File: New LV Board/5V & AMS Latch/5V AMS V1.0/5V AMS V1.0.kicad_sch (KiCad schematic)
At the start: 16 parts, among them J2 B12B-PH-K-S, J4 691137710002, K2 A161CS12VDC.64, K3 A161CS12VDC.64, K4 A161CS12VDC.64, SW1 Test Reset AMS, U1 LT1117-5.0

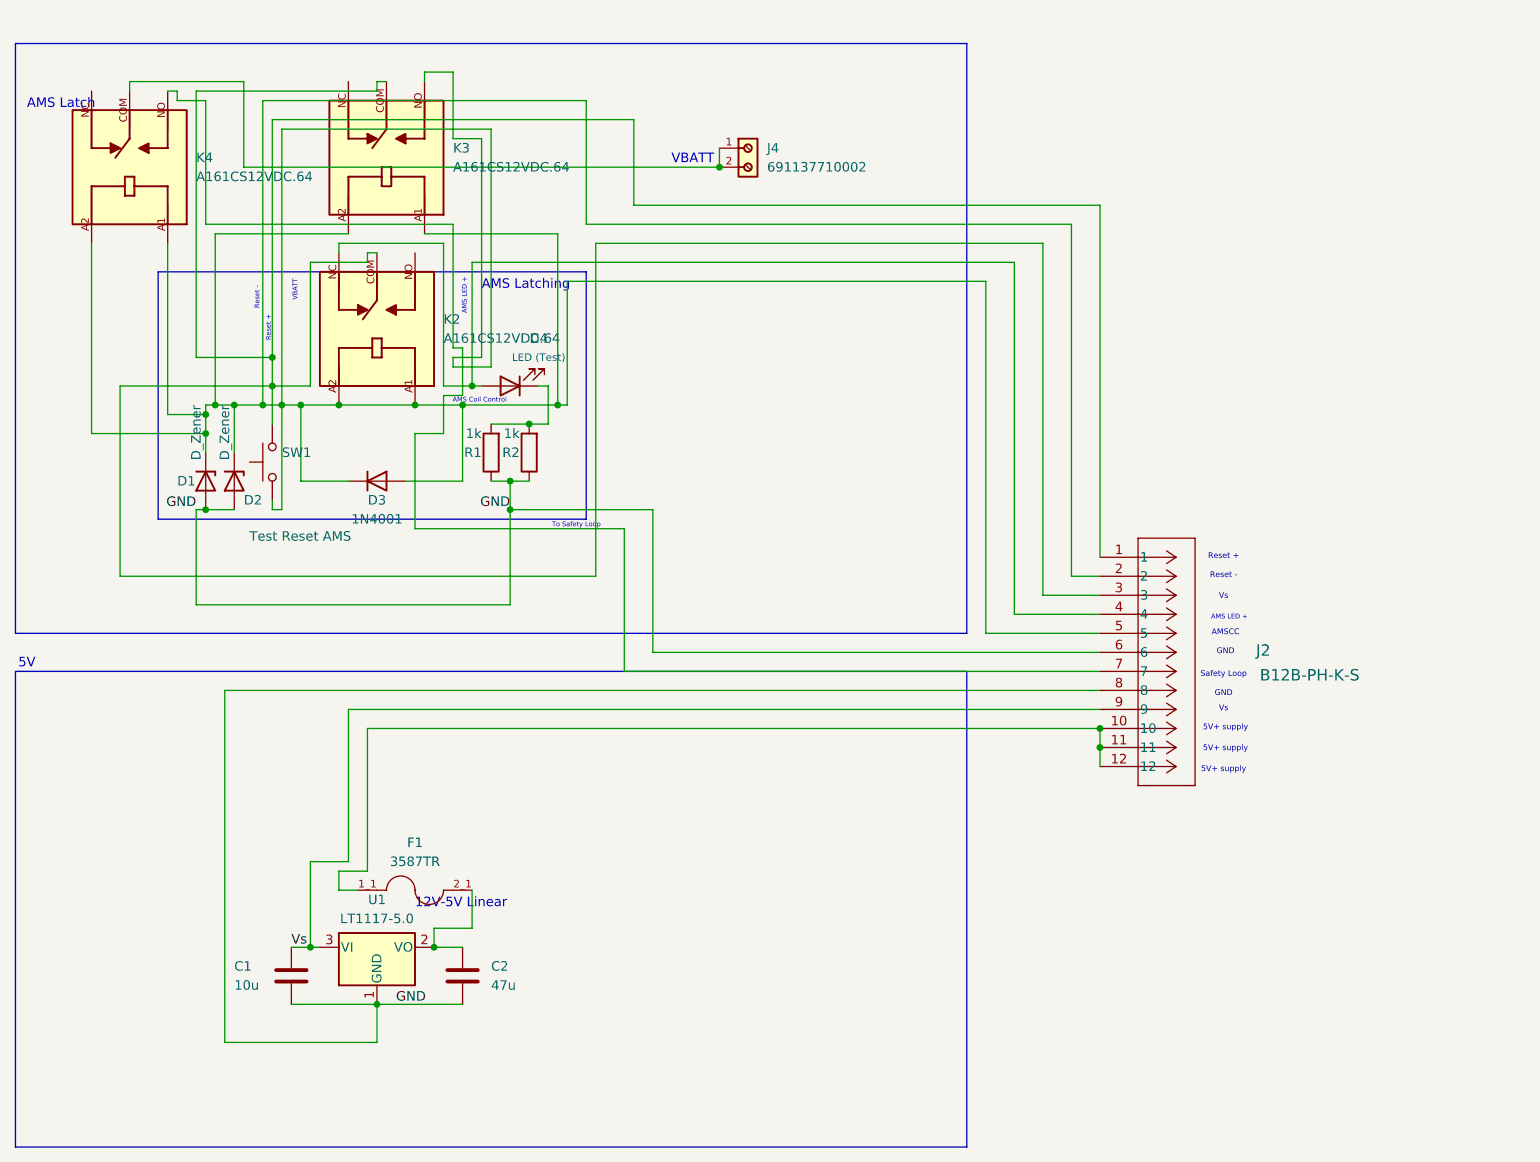
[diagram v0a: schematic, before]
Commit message: cleaned up schematics
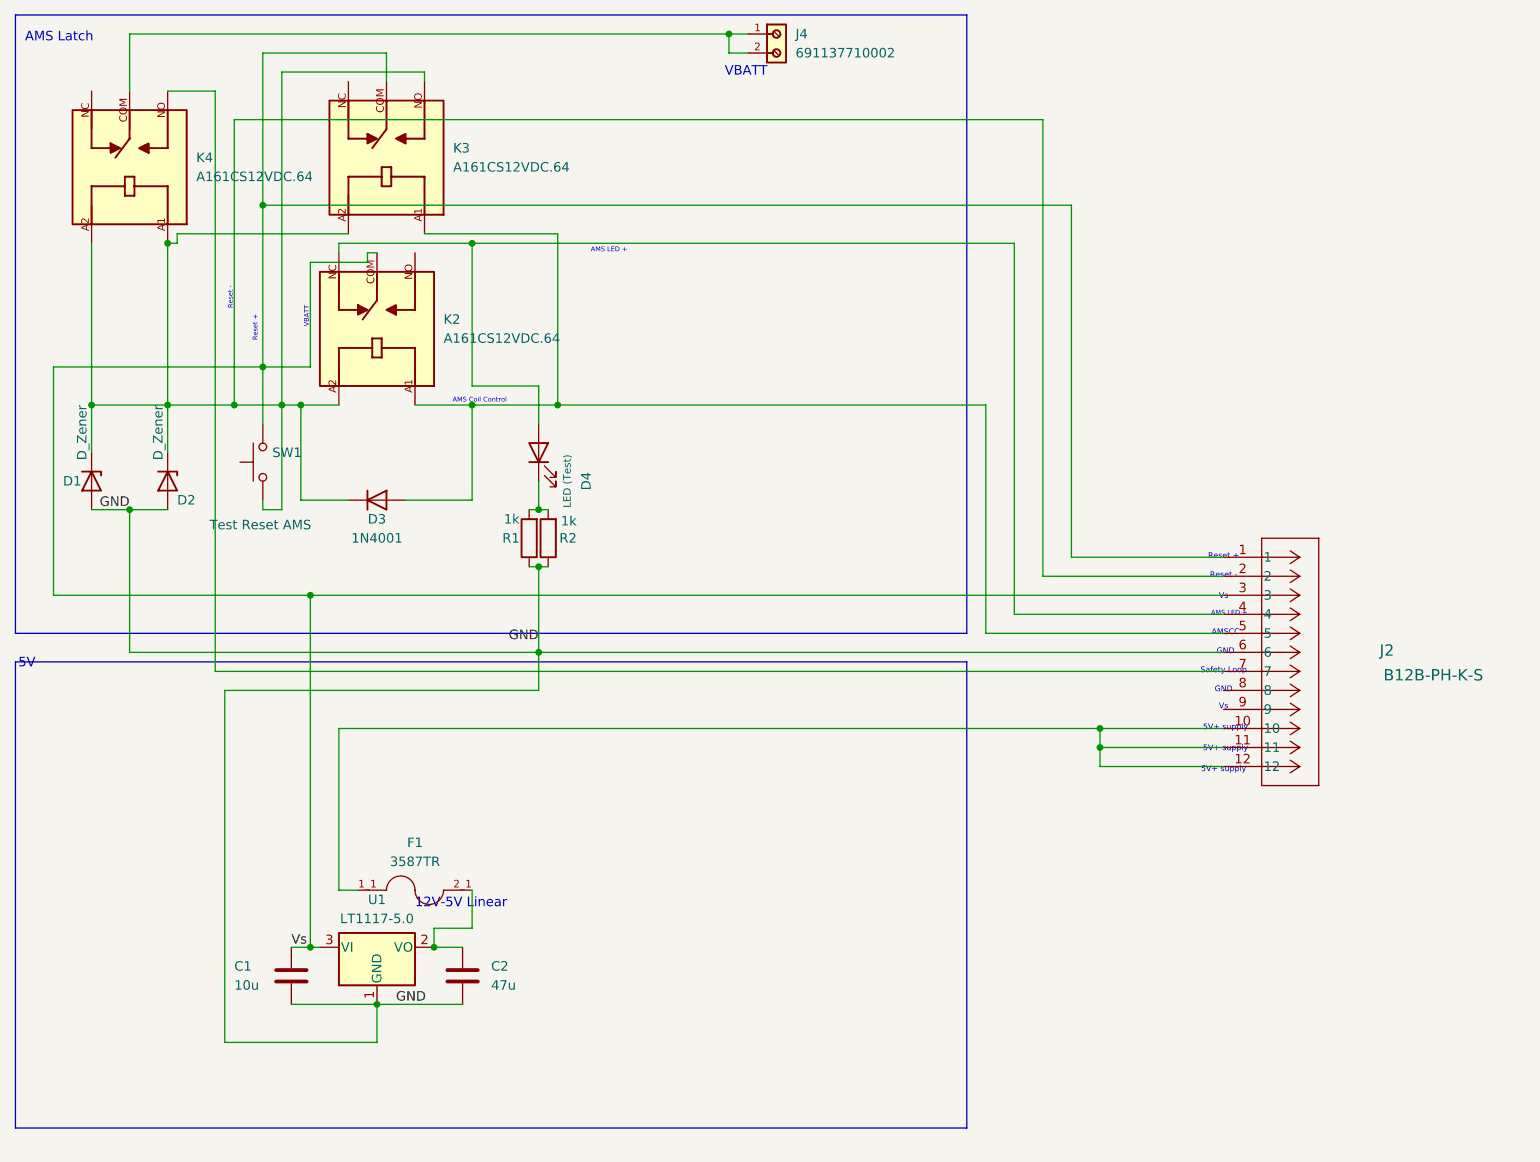
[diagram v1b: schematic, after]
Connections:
- net GND: no longer J2.8
- net Vs: now also J2.1, J2.3, K2.COM, K3.COM, SW1.2; no longer J2.9
- net at D1.1 (K), D2.1 (K), D3.1 (K)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: no longer D3.2 (A), J2.5, K2.A1, K3.A1
- new net: D3.2 (A), J2.5, K2.A1, K3.A1
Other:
- note removed: "AMS Latching"
- note removed: "To Safety Loop"
- moved on the sheet: D1, D2, D3, D4, J2, J4, R1, R2, SW1
